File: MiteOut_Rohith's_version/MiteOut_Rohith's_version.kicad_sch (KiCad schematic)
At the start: 28 parts, among them J1 JST, U1 ESP32-S3-WROOM-1, U2 INA260, U3 BQ25185DLHR, U4 TPS61022

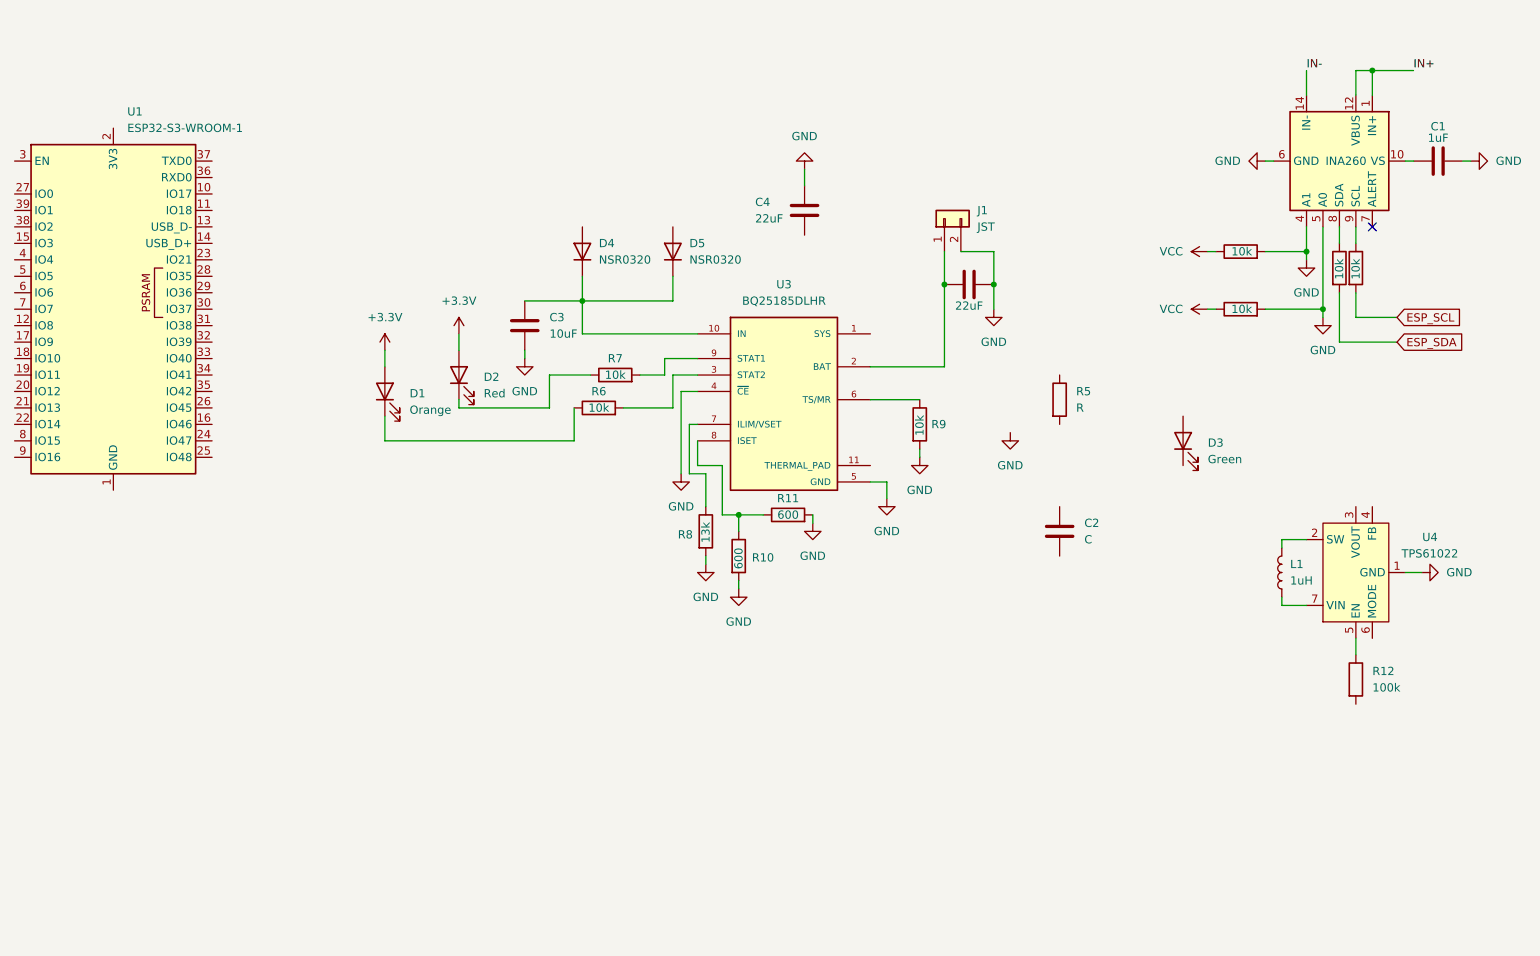
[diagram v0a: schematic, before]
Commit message: finished batt board
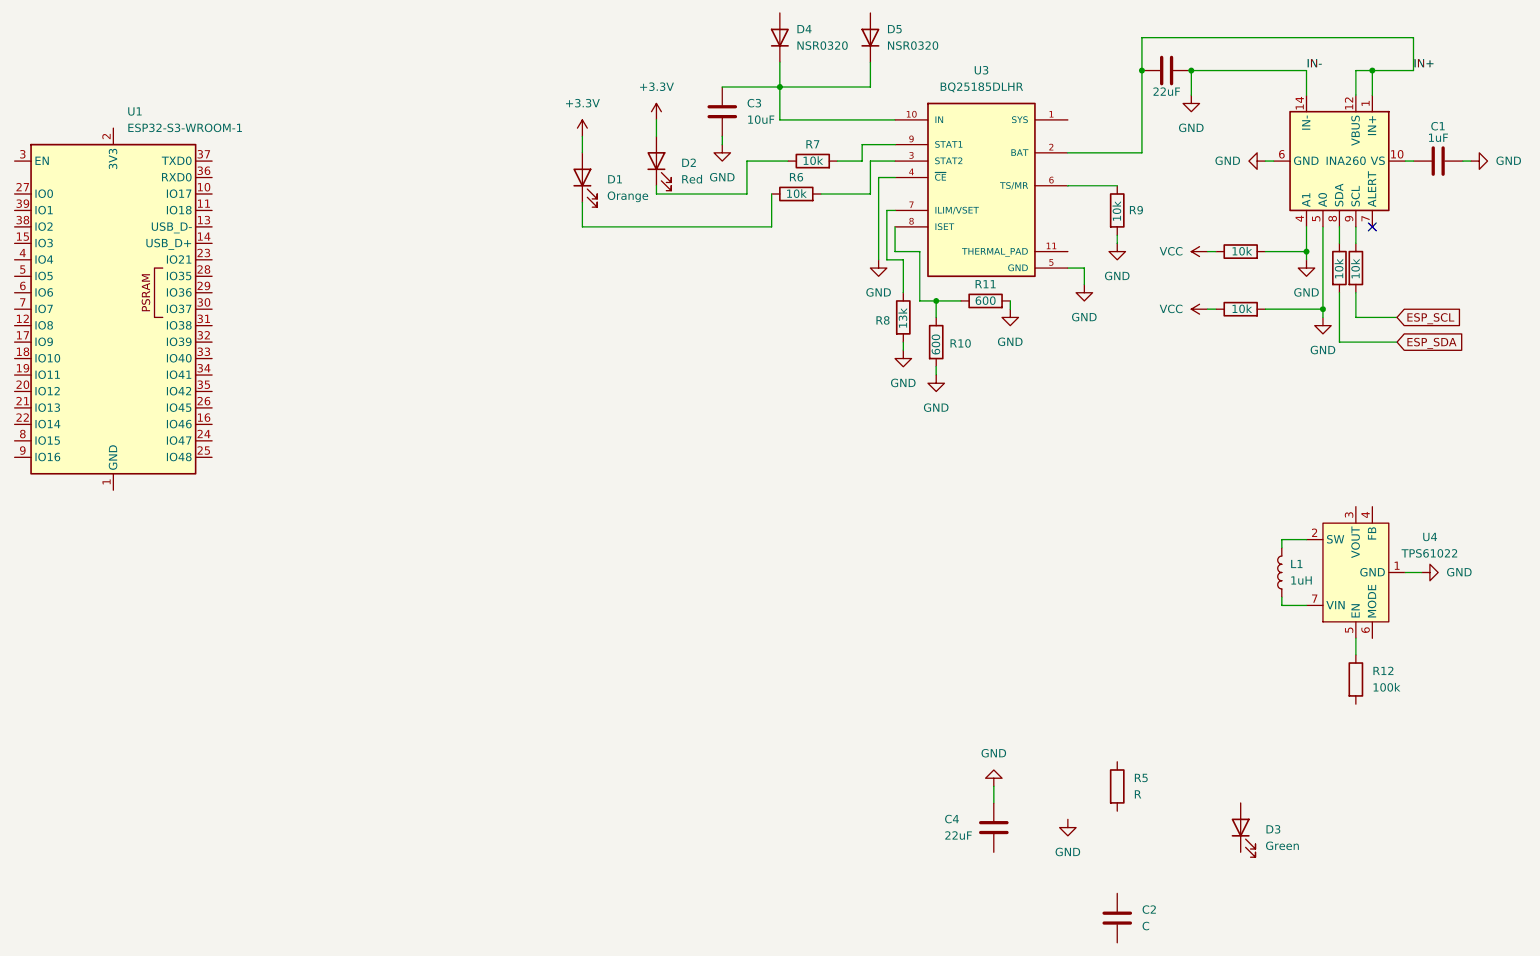
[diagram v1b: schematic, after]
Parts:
- removed J1: JST, Connector_JST:JST_XH_S2B-XH-A_1x02_P2.50mm_Horizontal, symbol Connector_Generic:Conn_01x02
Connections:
- net IN- is gone; now on net GND: U2.14 (IN-), U2.15 (IN-), U2.16 (IN-)
- net IN+: now also C5.1, U3.2 (BAT)
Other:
- moved on the sheet: C2, C3, C4, D1, D2, D3, D4, D5, R10, R11, R5, R6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
